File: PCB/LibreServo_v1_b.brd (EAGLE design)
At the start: 43.5 x 64.5 mm, 126 parts

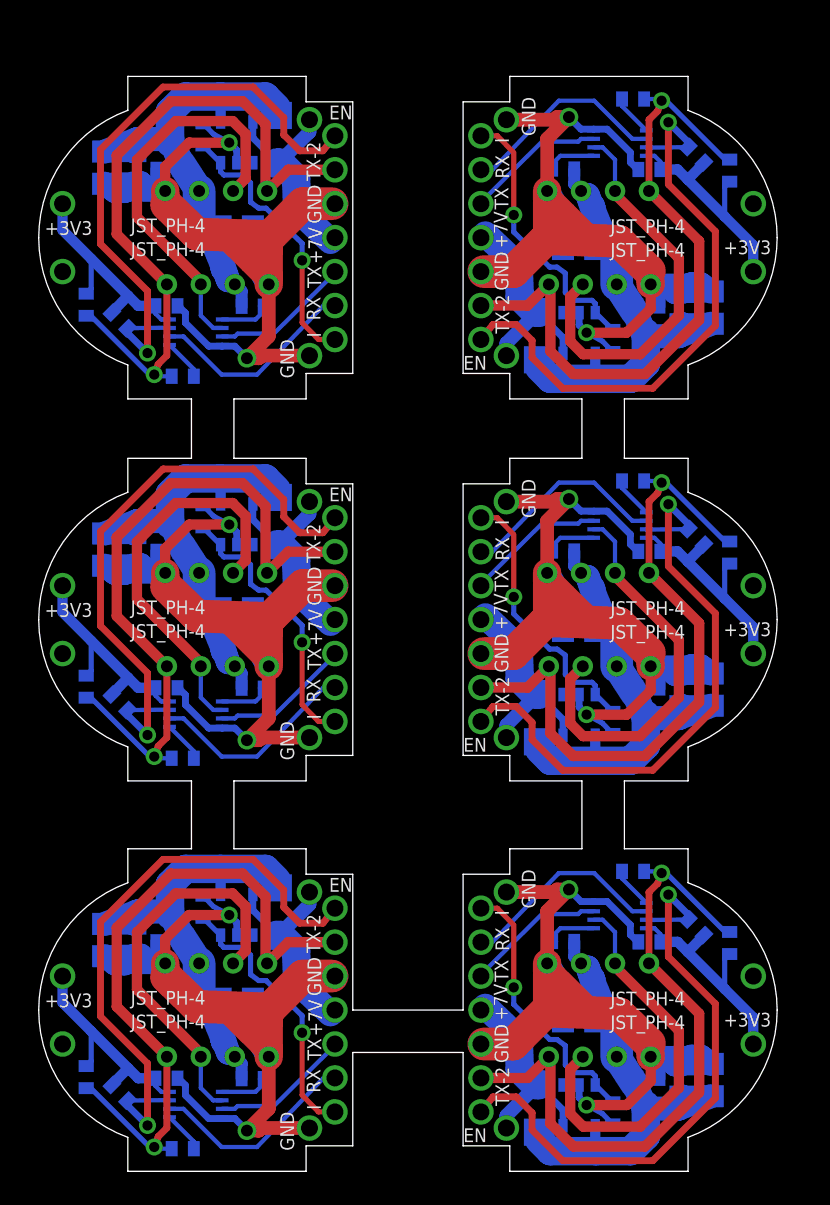
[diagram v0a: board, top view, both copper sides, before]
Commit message: LibreServo v1.c
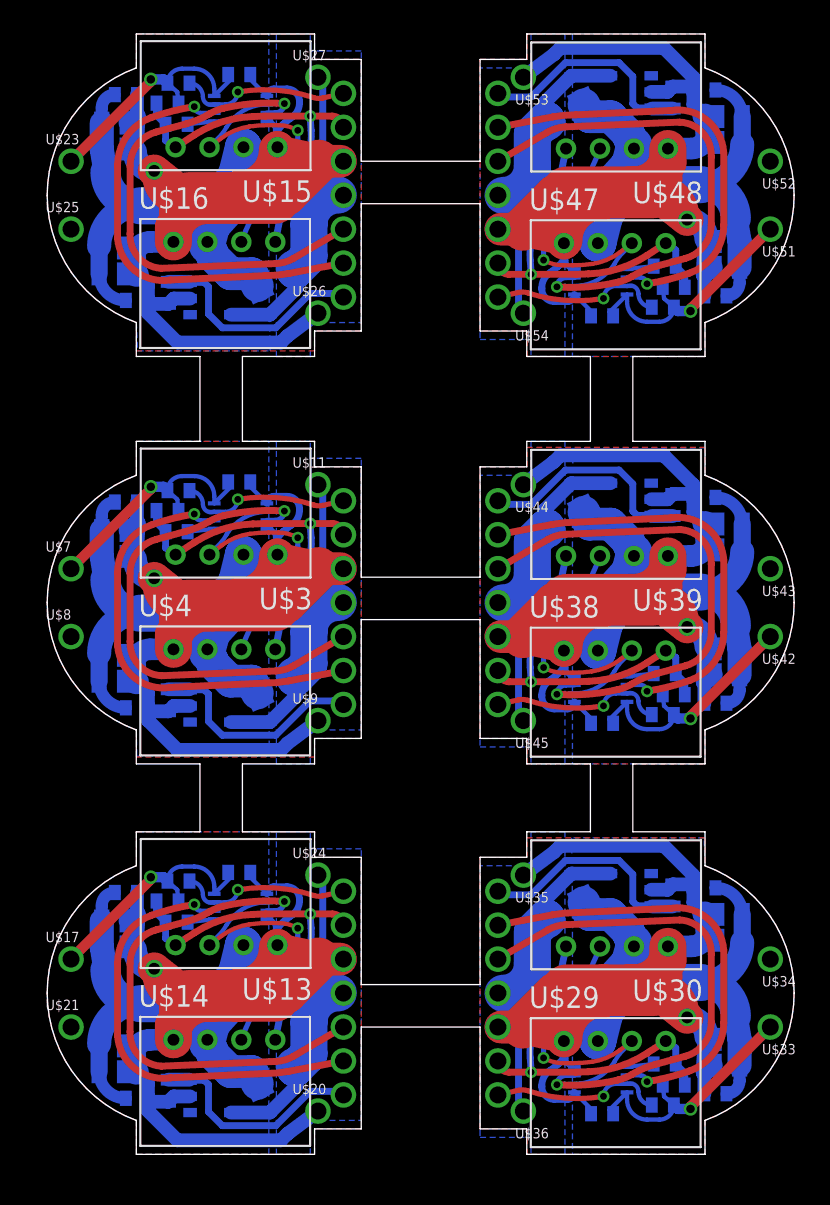
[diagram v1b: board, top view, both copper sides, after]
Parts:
- C11, C12, C16, C17, C18, C19, C20, C21, C25, C26, C27, C28, C32, C33, C34, C35, C39, C4, C40, C41, C42, C5, C6, C7: value 10uF -> 22uF; device rcl:C0805 -> Propio:0805_MIN
- R1, R16, R21, R26, R3, R8: device rcl:R1206 -> Propio:1206_ESTRECHA
- R12, R14, R19, R24, R29, R6: value 160 -> 100
- R13, R15, R20, R25, R30, R7: value 10K -> 100K
- R17, R2, R22, R27, R4, R9: value 160 -> 1k1
- moved U$23 49.6 mm to (1.90, 59.5), turned to 0 degrees
- moved U$42 48.9 mm to (43.1, 31.5), turned to 180 degrees
- moved C17 48.5 mm to (4.46, 61.7), turned to 180 degrees
- moved U$15 48.4 mm to (16.0, 66.6), flipped to the top, turned to 180 degrees
- moved C33 47.3 mm to (40.5, 29.3), turned to 0 degrees
- moved C8 46.6 mm to (5.14, 63.4), turned to 180 degrees
- moved C16 46.2 mm to (4.46, 60.2), turned to 180 degrees
- moved U$38 46.0 mm to (29.0, 24.4), flipped to the top, turned to 0 degrees
- moved U$25 45.3 mm to (1.90, 55.5), turned to 0 degrees
- moved U$43 45.2 mm to (43.1, 35.5), turned to 180 degrees
- moved C29 45.1 mm to (39.9, 27.6), turned to 0 degrees
- moved C32 45.0 mm to (40.5, 30.8), turned to 0 degrees
- moved R15 42.4 mm to (7.59, 62.9), turned to 180 degrees
- moved R25 41.5 mm to (37.4, 28.1), turned to 0 degrees
- moved R10 40.6 mm to (8.23, 64.1), turned to 180 degrees
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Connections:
- net +7V_2_CABLE: now also C11.1, C12.1, C13.1, C14.1, C20.1, C21.1; no longer C11.2, C12.2, C13.2, C14.2, C20.2, C21.2
- net +7V_2_CABLE1: now also C1.1, C2.1, C4.1, C5.1, C6.1, C7.1; no longer C1.2, C2.2, C4.2, C5.2, C6.2, C7.2
- net +7V_2_CABLE2: now also C16.1, C17.1, C18.1, C19.1, C8.1, C9.1; no longer C16.2, C17.2, C18.2, C19.2, C8.2, C9.2
- net +7V_2_CABLE3: now also C22.1, C23.1, C25.1, C26.1, C27.1, C28.1; no longer C22.2, C23.2, C25.2, C26.2, C27.2, C28.2
- net +7V_2_CABLE4: now also C29.1, C30.1, C32.1, C33.1, C34.1, C35.1; no longer C29.2, C30.2, C32.2, C33.2, C34.2, C35.2
- net +7V_2_CABLE5: now also C36.1, C37.1, C39.1, C40.1, C41.1, C42.1; no longer C36.2, C37.2, C39.2, C40.2, C41.2, C42.2
- net GND1: now also C1.2, C2.2, C4.2, C5.2, C6.2, C7.2; no longer C1.1, C2.1, C4.1, C5.1, C6.1, C7.1
- net GND2: now also C11.2, C12.2, C13.2, C14.2, C20.2, C21.2; no longer C11.1, C12.1, C13.1, C14.1, C20.1, C21.1
- net GND3: now also C16.2, C17.2, C18.2, C19.2, C8.2, C9.2; no longer C16.1, C17.1, C18.1, C19.1, C8.1, C9.1
- net GND4: now also C22.2, C23.2, C25.2, C26.2, C27.2, C28.2; no longer C22.1, C23.1, C25.1, C26.1, C27.1, C28.1
- net GND5: now also C29.2, C30.2, C32.2, C33.2, C34.2, C35.2; no longer C29.1, C30.1, C32.1, C33.1, C34.1, C35.1
- net GND6: now also C36.2, C37.2, C39.2, C40.2, C41.2, C42.2; no longer C36.1, C37.1, C39.1, C40.1, C41.1, C42.1
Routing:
- net EN_SERIAL_6: track 35.5 -> 9.89 mm
- net EN_SERIAL_4: track 35.5 -> 9.89 mm
- net EN_SERIAL_3: track 35.5 -> 9.89 mm
- net EN_SERIAL_5: track 35.5 -> 9.89 mm
- net EN_SERIAL_1: track 35.5 -> 9.89 mm
- net EN_SERIAL_2: track 35.5 -> 9.89 mm
- net TX_2: track 8.27 -> 29.6 mm, vias 0 -> 1
- net TX_1: track 8.27 -> 29.6 mm, vias 0 -> 1
- net TX_4: track 8.27 -> 29.6 mm, vias 0 -> 1
- net TX_3: track 8.27 -> 29.6 mm, vias 0 -> 1
- net TX_6: track 8.27 -> 29.6 mm, vias 0 -> 1
- net TX_5: track 8.27 -> 29.6 mm, vias 0 -> 1
- net TX_2_CABLE3: track 40.0 -> 21.5 mm
- net TX_2_CABLE2: track 40.0 -> 21.5 mm
- net TX_2_CABLE5: track 40.0 -> 21.5 mm
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- added copper zone on layer 16, net +7V_1
- added copper zone on layer 16, net +7V_2
- added copper zone on layer 16, net +7V_2_CABLE
- added copper zone on layer 16, net +7V_2_CABLE1
- added copper zone on layer 16, net +7V_2_CABLE2
- added copper zone on layer 16, net +7V_2_CABLE3
- added copper zone on layer 16, net +7V_2_CABLE4
- added copper zone on layer 16, net +7V_2_CABLE5
- added copper zone on layer 16, net +7V_3
- added copper zone on layer 16, net +7V_4
- added copper zone on layer 16, net +7V_5
- added copper zone on layer 16, net +7V_6
- added copper zone on layer 1, net GND1
- added copper zone on layer 1, net GND2
- added copper zone on layer 1, net GND3
- added copper zone on layer 1, net GND4
- added copper zone on layer 1, net GND5
- added copper zone on layer 1, net GND6
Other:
- board size 43.5 x 64.5 mm -> 44 x 66 mm
- board text added: "2x"
- board text added: "LibreServo v1.c"
- board text added: "SN74LVC2"
- board text removed: "JST_PH-4"
